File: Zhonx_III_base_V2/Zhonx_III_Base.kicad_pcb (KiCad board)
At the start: 4 copper layers, 48 x 32 mm, 50 parts, among them P100 CONN_BASE, P101 CONN_01X03, U101 MAX1607, U102 LT1370, U103 LP2992, U104 STM32F102C8, X101 8MHz

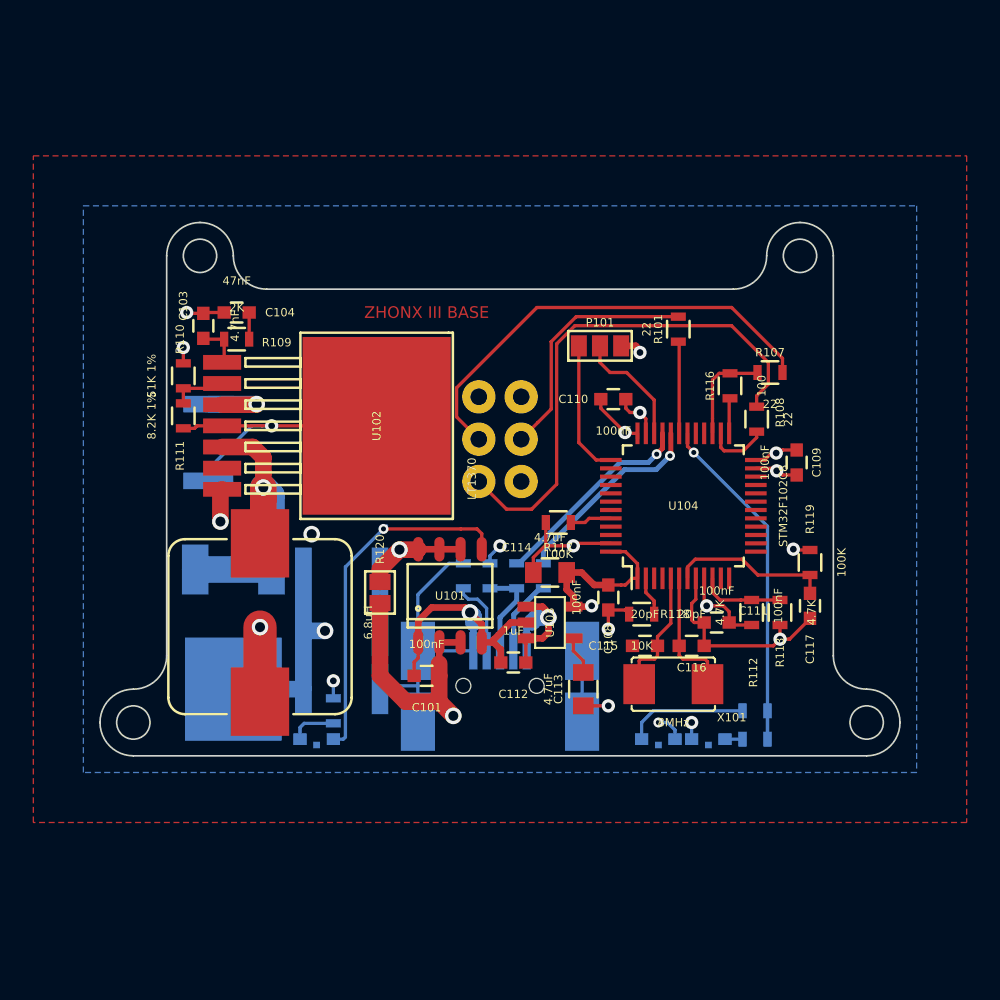
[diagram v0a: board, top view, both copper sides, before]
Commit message: Update Base_V2 (CamBam DXF)
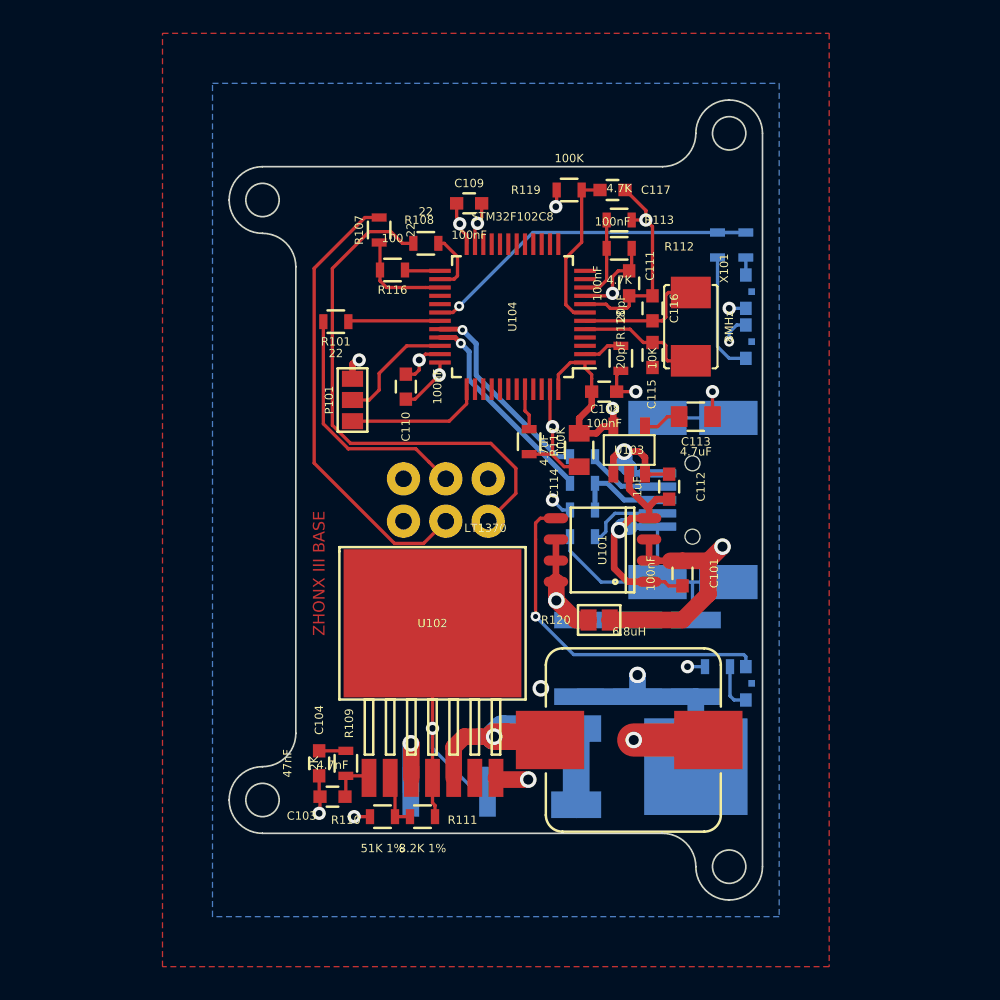
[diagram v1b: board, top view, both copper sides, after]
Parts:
- moved R114 29.7 mm to (119.2, 125.8), turned to 270 degrees
- moved C103 29.3 mm to (94.5, 158.9), turned to 180 degrees
- moved R110 29.0 mm to (97.5, 160.2), turned to 0 degrees
- moved D102 28.1 mm to (116.2, 157.2), turned to 90 degrees
- moved R115 28.0 mm to (117.5, 125.8), turned to 270 degrees
- moved R111 28.0 mm to (99.8, 160.2), turned to 0 degrees
- moved C117 27.6 mm to (111.2, 122.5), turned to 0 degrees
- moved C104 27.5 mm to (93.7, 156.9), turned to 270 degrees
- moved D103 26.9 mm to (119.2, 128.7), turned to 90 degrees
- moved R119 26.6 mm to (108.7, 122.5), turned to 180 degrees
- moved R109 26.3 mm to (95.2, 156.9), turned to 270 degrees
- moved D101 26.0 mm to (119.2, 152.2), turned to 90 degrees
- moved R113 25.5 mm to (111.7, 124.3), turned to 180 degrees
- moved C102 25.5 mm to (101.5, 158.7), turned to 0 degrees
- moved C109 25.1 mm to (102.7, 123.3), turned to 0 degrees
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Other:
- board size 48 x 32 mm -> 32 x 48 mm
